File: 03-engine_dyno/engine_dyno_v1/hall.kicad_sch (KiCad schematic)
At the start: 6 parts, among them J7 Screw_Terminal_01x03, U16 74LVC1G17

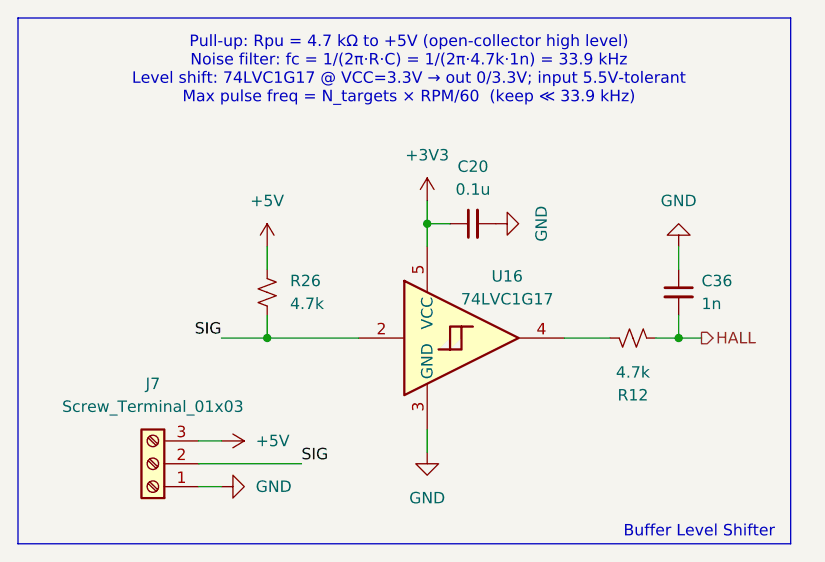
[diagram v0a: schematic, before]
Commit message: general layout
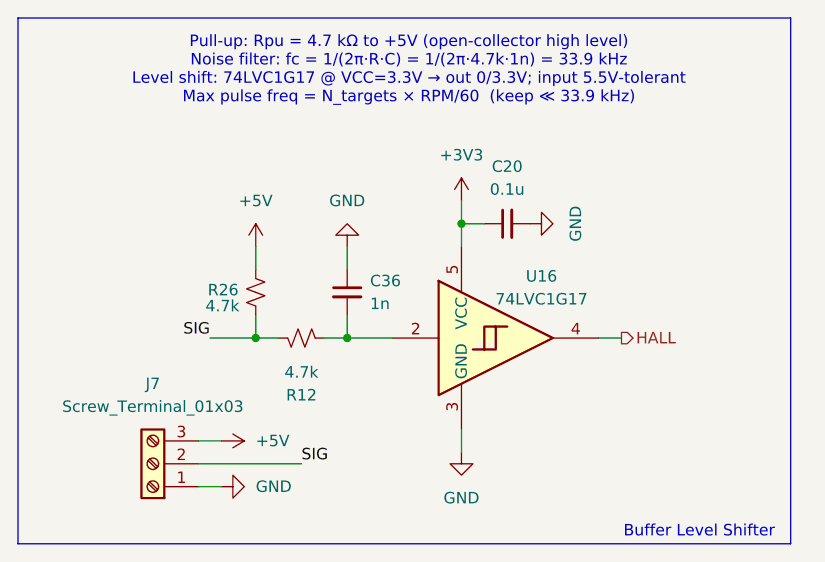
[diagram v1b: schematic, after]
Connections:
- net HALL: now also U16.4; no longer C36.2, R12.2
- net SIG: now also R12.1; no longer U16.2
- new net: C36.2, R12.2, U16.2
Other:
- moved on the sheet: C20, C36, R12, R26, U16
